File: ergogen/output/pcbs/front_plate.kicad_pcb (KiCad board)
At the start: 2 copper layers, 71.2 x 109.2 mm, 0 parts

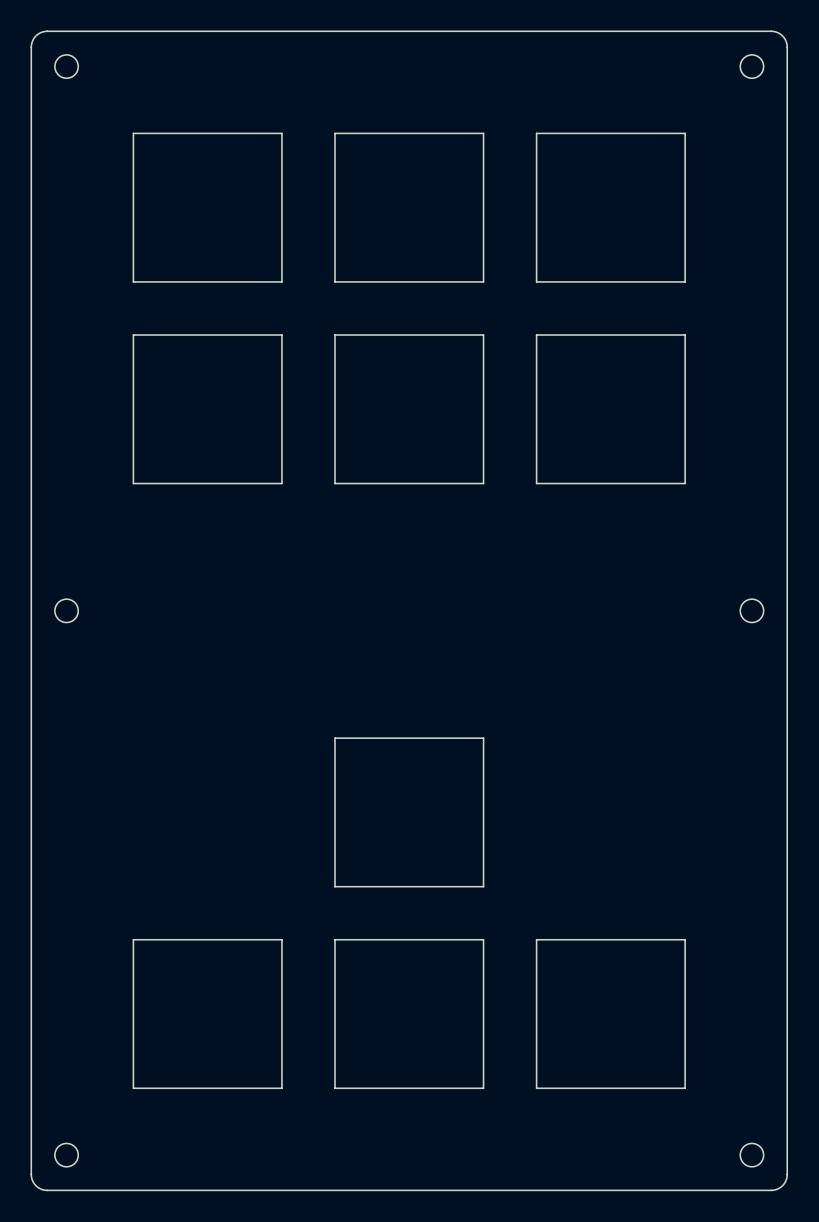
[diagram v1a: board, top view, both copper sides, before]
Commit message: Update assets
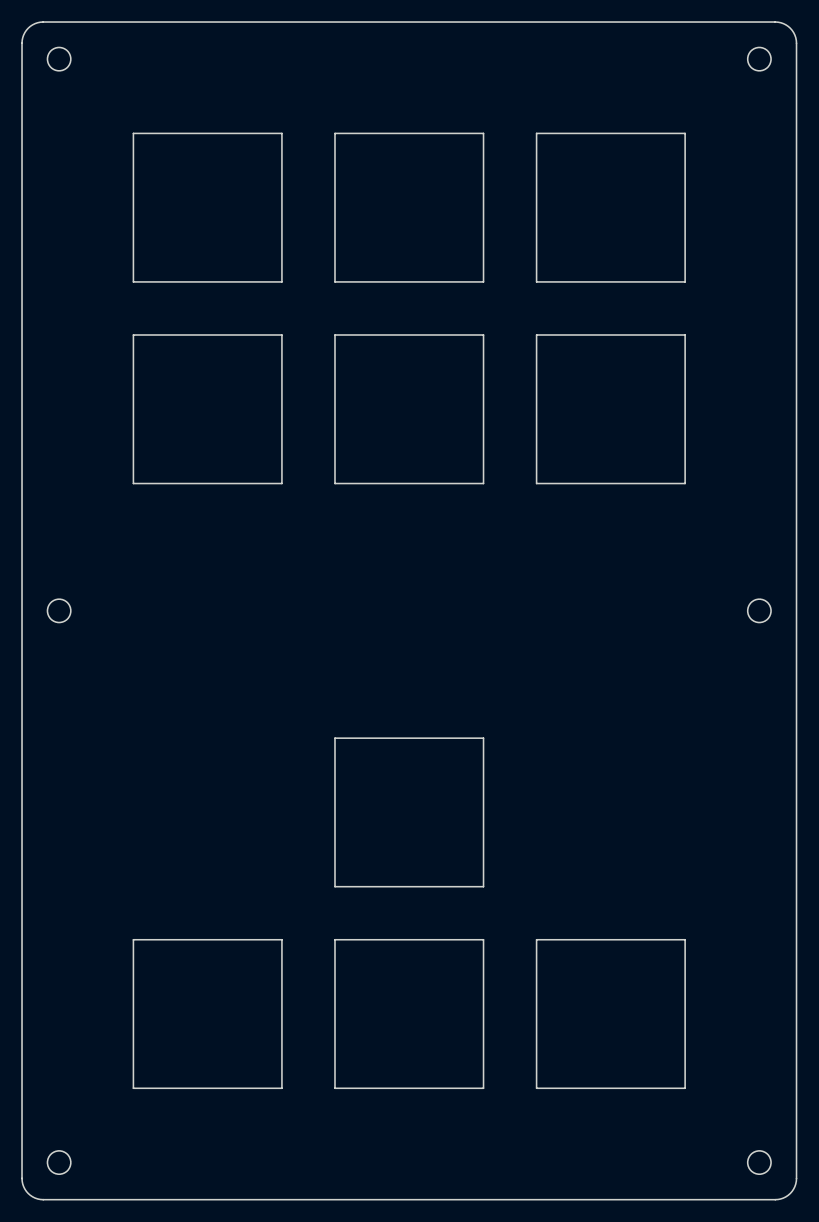
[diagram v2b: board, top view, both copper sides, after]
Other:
- board size 71.2 x 109.2 mm -> 73 x 111 mm
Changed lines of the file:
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@@
     (add_net "")
   )
-            (gr_line (start 44.875 141.625) (end 113.125 141.625) (angle 90) (layer Edge.Cuts) (width 0.15))
-(gr_line (start 114.625 140.125) (end 114.625 33.875) (angle 90) (layer Edge.Cuts) (width 0.15))
-(gr_line (start 113.125 32.375) (end 44.875 32.375) (angle 90) (layer Edge.Cuts) (width 0.15))
-(gr_line (start 43.375 33.875) (end 43.375 140.125) (angle 90) (layer Edge.Cuts) (width 0.15))
-(gr_arc (start 113.125 140.125) (end 113.125 141.625) (angle -90) (layer Edge.Cuts) (width 0.15))
-(gr_arc (start 113.125 33.875) (end 114.625 33.875) (angle -90) (layer Edge.Cuts) (width 0.15))
-(gr_arc (start 44.875 33.875) (end 44.875 32.375) (angle -90) (layer Edge.Cuts) (width 0.15))
-(gr_arc (start 44.875 140.125) (end 43.375 140.125) (angle -90) (layer Edge.Cuts) (width 0.15))
+            (gr_line (start 44.5 142.5) (end 113.5 142.5) (angle 90) (layer Edge.Cuts) (width 0.15))
+(gr_line (start 115.5 140.5) (end 115.5 33.5) (angle 90) (layer Edge.Cuts) (width 0.15))
+(gr_line (start 44.5 31.5) (end 113.5 31.5) (angle 90) (layer Edge.Cuts) (width 0.15))
+(gr_line (start 42.5 140.5) (end 42.5 33.5) (angle 90) (layer Edge.Cuts) (width 0.15))
+(gr_arc (start 113.5 140.5) (end 113.5 142.5) (angle -90) (layer Edge.Cuts) (width 0.15))
+(gr_arc (start 113.5 33.5) (end 115.5 33.5) (angle -90) (layer Edge.Cuts) (width 0.15))
+(gr_arc (start 44.5 33.5) (end 44.5 31.5) (angle -90) (layer Edge.Cuts) (width 0.15))
+(gr_arc (start 44.5 140.5) (end 42.5 140.5) (angle -90) (layer Edge.Cuts) (width 0.15))
 (gr_line (start 53 132) (end 67 132) (angle 90) (layer Edge.Cuts) (width 0.15))
 (gr_line (start 67 132) (end 67 118) (angle 90) (layer Edge.Cuts) (width 0.15))
@@
 (gr_line (start 105 42) (end 91 42) (angle 90) (layer Edge.Cuts) (width 0.15))
 (gr_line (start 91 42) (end 91 56) (angle 90) (layer Edge.Cuts) (width 0.15))
-(gr_circle (center 46.7 35.7) (end 47.800000000000004 35.7) (layer Edge.Cuts) (width 0.15))
-(gr_circle (center 111.3 35.7) (end 112.39999999999999 35.7) (layer Edge.Cuts) (width 0.15))
-(gr_circle (center 46.7 87) (end 47.800000000000004 87) (layer Edge.Cuts) (width 0.15))
-(gr_circle (center 111.3 87) (end 112.39999999999999 87) (layer Edge.Cuts) (width 0.15))
-(gr_circle (center 46.7 138.3) (end 47.800000000000004 138.3) (layer Edge.Cuts) (width 0.15))
-(gr_circle (center 111.3 138.3) (end 112.39999999999999 138.3) (layer Edge.Cuts) (width 0.15))
+(gr_circle (center 46 35) (end 47.1 35) (layer Edge.Cuts) (width 0.15))
+(gr_circle (center 112 35) (end 113.1 35) (layer Edge.Cuts) (width 0.15))
+(gr_circle (center 46 87) (end 47.1 87) (layer Edge.Cuts) (width 0.15))
+(gr_circle (center 112 87) (end 113.1 87) (layer Edge.Cuts) (width 0.15))
+(gr_circle (center 46 139) (end 47.1 139) (layer Edge.Cuts) (width 0.15))
+(gr_circle (center 112 139) (end 113.1 139) (layer Edge.Cuts) (width 0.15))
 )
